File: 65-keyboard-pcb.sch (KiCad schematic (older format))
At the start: 153 parts, among them J1 USB4085-GF-A_REVA, SW1 SW_PUSH, U1 ATmega32U4-AU, X1 XTAL_GND

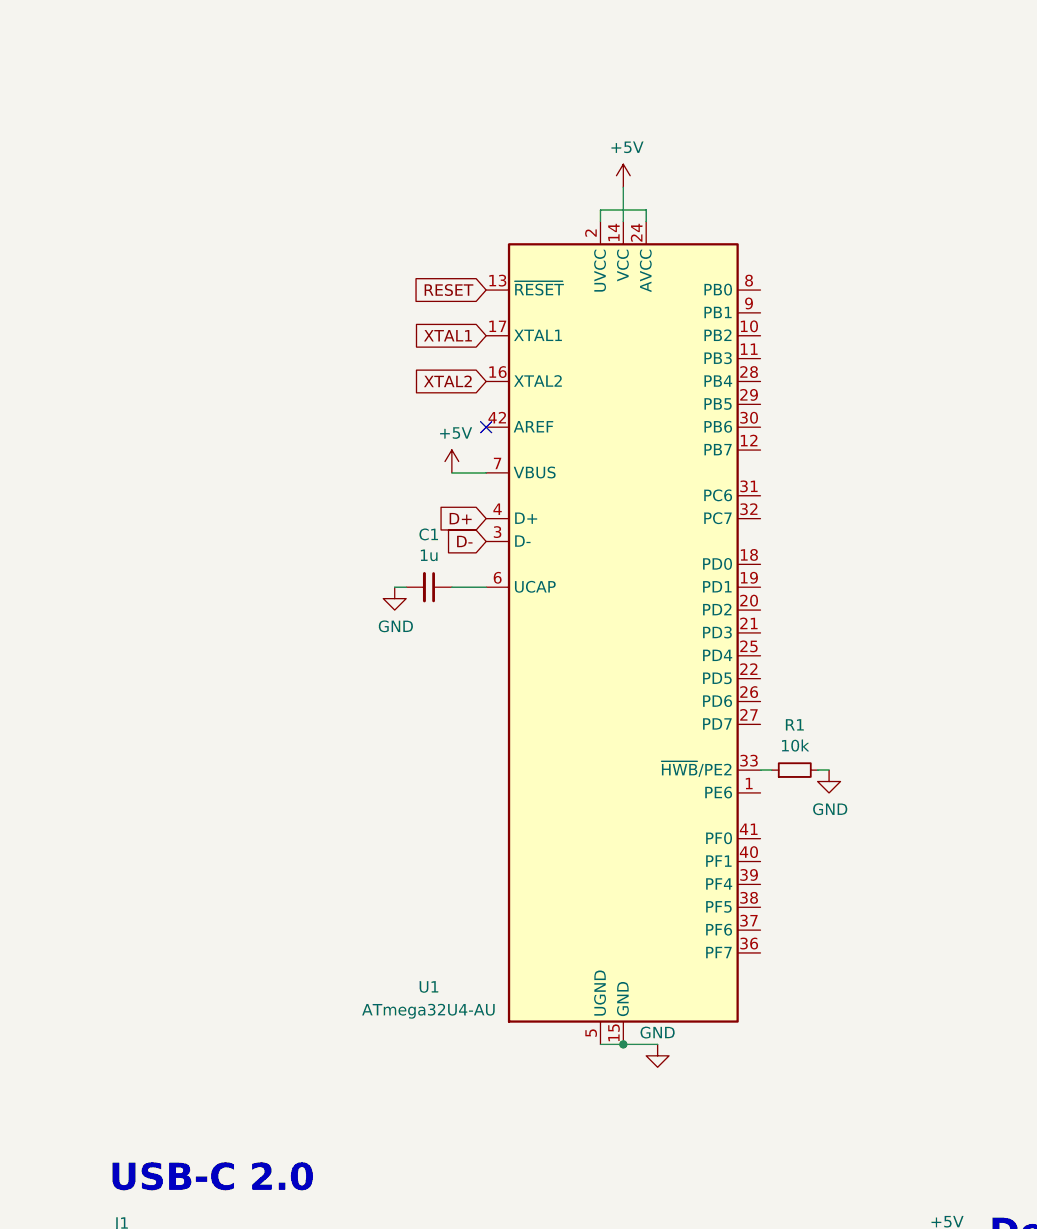
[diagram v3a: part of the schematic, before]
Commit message: Component placement
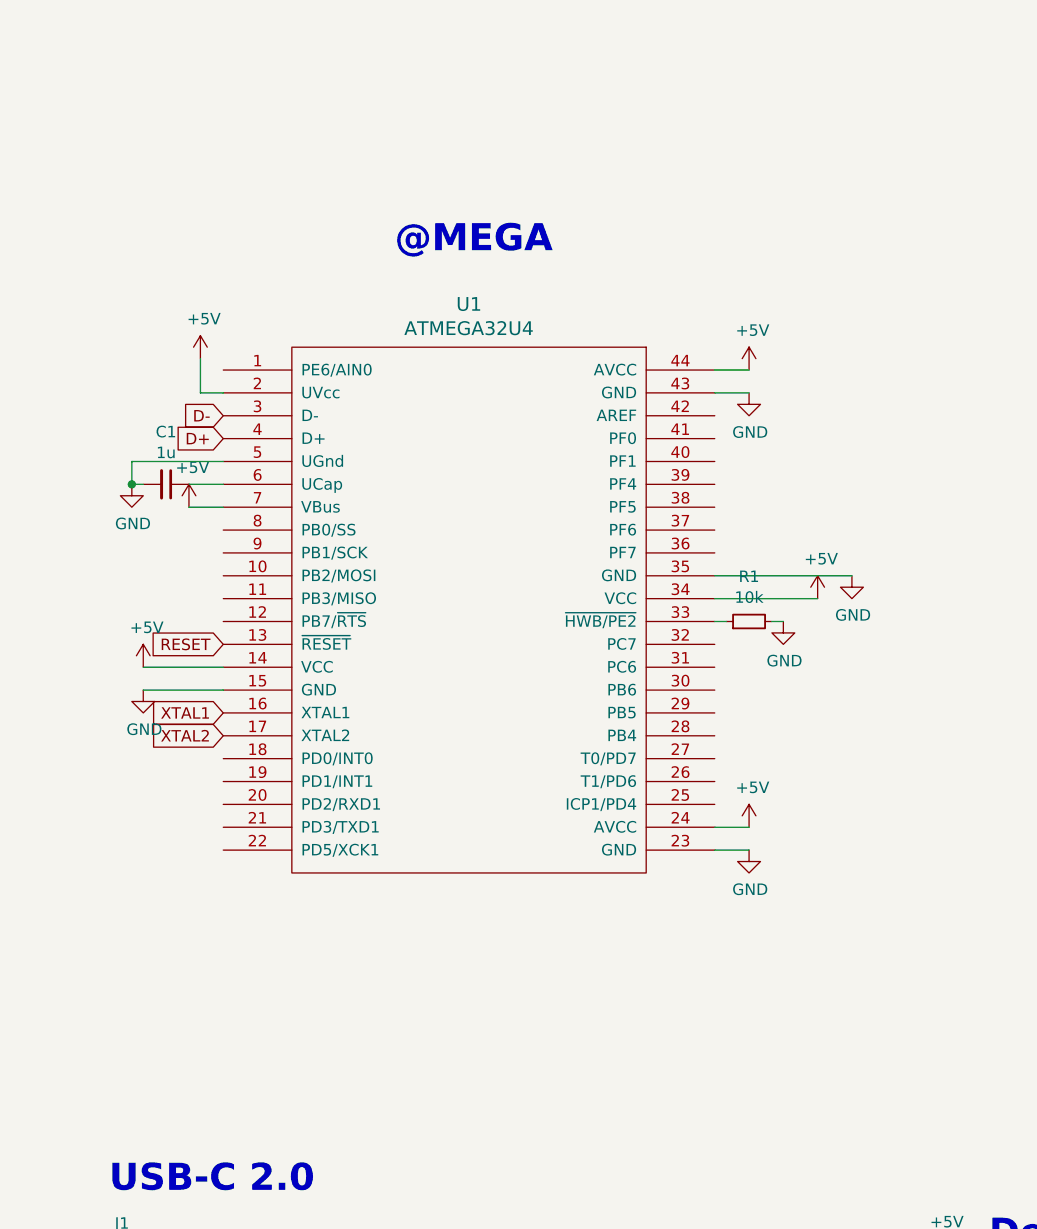
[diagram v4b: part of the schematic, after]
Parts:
- removed U1: ATmega32U4-AU, Package_QFP:TQFP-44_10x10mm_P0.8mm, symbol MCU_Microchip_ATmega:ATmega32U4-AU
- added U1: ATMEGA32U4, Package_QFP:TQFP-44_10x10mm_P0.8mm, symbol keyboard_parts:ATMEGA32U4
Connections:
- net +5V: now also U1.14 (VCC), U1.2 (UVcc), U1.24 (AVCC), U1.34 (VCC), U1.44 (AVCC), U1.7 (VBus)
- net D+: now also U1.4 (D+)
- net D-: now also U1.3 (D-)
- net GND: now also U1.15 (GND), U1.23 (GND), U1.35 (GND), U1.43 (GND), U1.5 (UGnd)
- net RESET: now also U1.13 (~RESET)
- net XTAL1: now also U1.16 (XTAL1)
- net XTAL2: now also U1.17 (XTAL2)
- net at R1.1: now also U1.33 (~HWB/PE2)
- net at C1.1: now also U1.6 (UCap)
- no-connect marks 3 -> 2
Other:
- note added: "@MEGA"
- moved on the sheet: C1, R1
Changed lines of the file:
@@
 Text GLabel 5600 4750 0    50   Input ~ 0
 ROW4
-$Comp
-L MCU_Microchip_ATmega:ATmega32U4-AU U1
-U 1 1 5F5682CF
-P 3450 3250
-F 0 "U1" H 2600 1700 50  0000 C CNN
-F 1 "ATmega32U4-AU" H 2600 1600 50  0000 C CNN
-F 2 "Package_QFP:TQFP-44_10x10mm_P0.8mm" H 3450 3250 50  0001 C CIN
-F 3 "http://ww1.microchip.com/downloads/en/DeviceDoc/Atmel-7766-8-bit-AVR-ATmega16U4-32U4_Datasheet.pdf" H 3450 3250 50  0001 C CNN
-	1    3450 3250
-	1    0    0    -1
-$EndComp
-Text GLabel 2850 1750 0    50   Input ~ 0
+Text GLabel 1700 3300 0    50   Input ~ 0
 RESET
 Text GLabel 6050 7350 2    50   Input ~ 0
@@
 $EndComp
 $Comp
-L power:GND #PWR0103
-U 1 1 5F57B366
-P 3600 5050
-F 0 "#PWR0103" H 3600 4800 50  0001 C CNN
-F 1 "GND" H 3600 5100 50  0000 C CNN
-F 2 "" H 3600 5050 50  0001 C CNN
-F 3 "" H 3600 5050 50  0001 C CNN
-	1    3600 5050
-	1    0    0    -1
-$EndComp
-Wire Wire Line
-	3350 5050 3450 5050
-Connection ~ 3450 5050
-Wire Wire Line
-	3450 5050 3600 5050
-Wire Wire Line
-	3350 1450 3350 1400
-Wire Wire Line
-	3350 1400 3550 1400
-Wire Wire Line
-	3550 1400 3550 1450
-$Comp
 L power:+5V #PWR0104
 U 1 1 5F588B35
-P 3450 1300
-F 0 "#PWR0104" H 3450 1150 50  0001 C CNN
-F 1 "+5V" H 3465 1473 50  0000 C CNN
-F 2 "" H 3450 1300 50  0001 C CNN
-F 3 "" H 3450 1300 50  0001 C CNN
-	1    3450 1300
-	1    0    0    -1
-$EndComp
-Wire Wire Line
-	3450 1300 3450 1450
+P 1600 2050
+F 0 "#PWR0104" H 1600 1900 50  0001 C CNN
+F 1 "+5V" H 1615 2223 50  0000 C CNN
+F 2 "" H 1600 2050 50  0001 C CNN
+F 3 "" H 1600 2050 50  0001 C CNN
+	1    1600 2050
+	1    0    0    -1
+$EndComp
+Wire Wire Line
+	1600 2050 1600 2200
 $Comp
 L keyboard_parts:XTAL_GND X1
@@
 Text GLabel 4300 7000 1    50   Input ~ 0
 XTAL2
-Text GLabel 2850 1950 0    50   Input ~ 0
+Text GLabel 1700 3600 0    50   Input ~ 0
 XTAL1
-Text GLabel 2850 2150 0    50   Input ~ 0
+Text GLabel 1700 3700 0    50   Input ~ 0
 XTAL2
-NoConn ~ 2850 2350
 $Comp
 L power:+5V #PWR0106
 U 1 1 5F5B165B
-P 2700 2550
-F 0 "#PWR0106" H 2700 2400 50  0001 C CNN
-F 1 "+5V" H 2715 2723 50  0000 C CNN
-F 2 "" H 2700 2550 50  0001 C CNN
-F 3 "" H 2700 2550 50  0001 C CNN
-	1    2700 2550
-	1    0    0    -1
-$EndComp
-Wire Wire Line
-	2700 2550 2850 2550
-Text GLabel 2850 2750 0    50   Input ~ 0
+P 1550 2700
+F 0 "#PWR0106" H 1550 2550 50  0001 C CNN
+F 1 "+5V" H 1565 2873 50  0000 C CNN
+F 2 "" H 1550 2700 50  0001 C CNN
+F 3 "" H 1550 2700 50  0001 C CNN
+	1    1550 2700
+	1    0    0    -1
+$EndComp
+Wire Wire Line
+	1550 2700 1700 2700
+Text GLabel 1700 2400 0    50   Input ~ 0
 D+
-Text GLabel 2850 2850 0    50   Input ~ 0
+Text GLabel 1700 2300 0    50   Input ~ 0
 D-
 $Comp
 L Device:R_Small R1
 U 1 1 5F5B953F
-P 4200 3850
-F 0 "R1" V 4396 3850 50  0000 C CNN
-F 1 "10k" V 4305 3850 50  0000 C CNN
-F 2 "Resistor_SMD:R_0805_2012Metric_Pad1.15x1.40mm_HandSolder" H 4200 3850 50  0001 C CNN
-F 3 "~" H 4200 3850 50  0001 C CNN
-	1    4200 3850
+P 4000 3200
+F 0 "R1" V 4196 3200 50  0000 C CNN
+F 1 "10k" V 4105 3200 50  0000 C CNN
+F 2 "Resistor_SMD:R_0805_2012Metric_Pad1.15x1.40mm_HandSolder" H 4000 3200 50  0001 C CNN
+F 3 "~" H 4000 3200 50  0001 C CNN
+	1    4000 3200
 	0    -1   -1   0
 $EndComp
 Wire Wire Line
-	4100 3850 4050 3850
+	3900 3200 3850 3200
 $Comp
 L power:GND #PWR0107
 U 1 1 5F5C1E45
-P 4350 3850
-F 0 "#PWR0107" H 4350 3600 50  0001 C CNN
-F 1 "GND" H 4355 3677 50  0000 C CNN
-F 2 "" H 4350 3850 50  0001 C CNN
-F 3 "" H 4350 3850 50  0001 C CNN
-	1    4350 3850
-	1    0    0    -1
-$EndComp
-Wire Wire Line
-	4350 3850 4300 3850
+P 4150 3200
+F 0 "#PWR0107" H 4150 2950 50  0001 C CNN
+F 1 "GND" H 4155 3027 50  0000 C CNN
+F 2 "" H 4150 3200 50  0001 C CNN
+F 3 "" H 4150 3200 50  0001 C CNN
+	1    4150 3200
+	1    0    0    -1
+$EndComp
+Wire Wire Line
+	4150 3200 4100 3200
 $Comp
 L Device:C_Small C1
 U 1 1 5F5CAA76
-P 2600 3050
-F 0 "C1" V 2371 3050 50  0000 C CNN
-F 1 "1u" V 2462 3050 50  0000 C CNN
-F 2 "Capacitor_SMD:C_0805_2012Metric_Pad1.15x1.40mm_HandSolder" H 2600 3050 50  0001 C CNN
-F 3 "~" H 2600 3050 50  0001 C CNN
-	1    2600 3050
+P 1450 2600
+F 0 "C1" V 1221 2600 50  0000 C CNN
+F 1 "1u" V 1312 2600 50  0000 C CNN
+F 2 "Capacitor_SMD:C_0805_2012Metric_Pad1.15x1.40mm_HandSolder" H 1450 2600 50  0001 C CNN
+F 3 "~" H 1450 2600 50  0001 C CNN
+	1    1450 2600
 	0    1    1    0
 $EndComp
@@
 L power:GND #PWR0108
 U 1 1 5F5DFA66
-P 2450 3050
-F 0 "#PWR0108" H 2450 2800 50  0001 C CNN
-F 1 "GND" H 2455 2877 50  0000 C CNN
-F 2 "" H 2450 3050 50  0001 C CNN
-F 3 "" H 2450 3050 50  0001 C CNN
-	1    2450 3050
-	1    0    0    -1
-$EndComp
-Wire Wire Line
-	2450 3050 2500 3050
-Wire Wire Line
-	2700 3050 2850 3050
+P 1300 2600
+F 0 "#PWR0108" H 1300 2350 50  0001 C CNN
+F 1 "GND" H 1305 2427 50  0000 C CNN
+F 2 "" H 1300 2600 50  0001 C CNN
+F 3 "" H 1300 2600 50  0001 C CNN
+	1    1300 2600
+	1    0    0    -1
+$EndComp
+Wire Wire Line
+	1300 2600 1350 2600
+Wire Wire Line
+	1550 2600 1700 2600
 Text Notes 3700 6600 0    118  ~ 24
 Crystal
@@
 Wire Wire Line
 	10600 2100 10600 4350
+$Comp
+L keyboard_parts:ATMEGA32U4 U1
+U 1 1 5F56E3DD
+P 2750 3150
+F 0 "U1" H 2775 4487 60  0000 C CNN
+F 1 "ATMEGA32U4" H 2775 4381 60  0000 C CNN
+F 2 "Package_QFP:TQFP-44_10x10mm_P0.8mm" H 2750 3150 60  0001 C CNN
+F 3 "" H 2750 3150 60  0000 C CNN
+	1    2750 3150
+	1    0    0    -1
+$EndComp
+Wire Wire Line
+	1700 2200 1600 2200
+$Comp
+L power:+5V #PWR0103
+U 1 1 5F5A8F73
+P 1350 3400
+F 0 "#PWR0103" H 1350 3250 50  0001 C CNN
+F 1 "+5V" H 1365 3573 50  0000 C CNN
+F 2 "" H 1350 3400 50  0001 C CNN
+F 3 "" H 1350 3400 50  0001 C CNN
+	1    1350 3400
+	1    0    0    -1
+$EndComp
+$Comp
+L power:GND #PWR0116
+U 1 1 5F5AA002
+P 1350 3500
+F 0 "#PWR0116" H 1350 3250 50  0001 C CNN
+F 1 "GND" H 1355 3327 50  0000 C CNN
+F 2 "" H 1350 3500 50  0001 C CNN
+F 3 "" H 1350 3500 50  0001 C CNN
+	1    1350 3500
+	1    0    0    -1
+$EndComp
+Wire Wire Line
+	1350 3500 1700 3500
+Wire Wire Line
+	1700 3400 1350 3400
+Wire Wire Line
+	1700 2500 1300 2500
+Wire Wire Line
+	1300 2500 1300 2600
+Connection ~ 1300 2600
+Text Notes 2450 1600 0    118  ~ 24
+@MEGA
+$Comp
+L power:+5V #PWR?
+U 1 1 5F61FD1D
+P 4000 2100
+F 0 "#PWR?" H 4000 1950 50  0001 C CNN
+F 1 "+5V" H 4015 2273 50  0000 C CNN
+F 2 "" H 4000 2100 50  0001 C CNN
+F 3 "" H 4000 2100 50  0001 C CNN
+	1    4000 2100
+	1    0    0    -1
+$EndComp
+$Comp
+L power:GND #PWR?
+U 1 1 5F620425
+P 4000 2200
+F 0 "#PWR?" H 4000 1950 50  0001 C CNN
+F 1 "GND" H 4005 2027 50  0000 C CNN
+F 2 "" H 4000 2200 50  0001 C CNN
+F 3 "" H 4000 2200 50  0001 C CNN
+	1    4000 2200
+	1    0    0    -1
+$EndComp
+Wire Wire Line
+	4000 2200 3850 2200
+Wire Wire Line
+	4000 2100 3850 2100
+$Comp
+L power:GND #PWR?
+U 1 1 5F635EFD
+P 4450 3000
+F 0 "#PWR?" H 4450 2750 50  0001 C CNN
+F 1 "GND" H 4455 2827 50  0000 C CNN
+F 2 "" H 4450 3000 50  0001 C CNN
+F 3 "" H 4450 3000 50  0001 C CNN
+	1    4450 3000
+	1    0    0    -1
+$EndComp
+$Comp
+L power:+5V #PWR?
+U 1 1 5F636303
+P 4300 3100
+F 0 "#PWR?" H 4300 2950 50  0001 C CNN
+F 1 "+5V" H 4315 3273 50  0000 C CNN
+F 2 "" H 4300 3100 50  0001 C CNN
+F 3 "" H 4300 3100 50  0001 C CNN
+	1    4300 3100
+	1    0    0    -1
+$EndComp
+Wire Wire Line
+	4300 3100 3850 3100
+Wire Wire Line
+	3850 3000 4450 3000
+$Comp
+L power:+5V #PWR?
+U 1 1 5F64C6D1
+P 4000 4100
+F 0 "#PWR?" H 4000 3950 50  0001 C CNN
+F 1 "+5V" H 4015 4273 50  0000 C CNN
+F 2 "" H 4000 4100 50  0001 C CNN
+F 3 "" H 4000 4100 50  0001 C CNN
+	1    4000 4100
+	1    0    0    -1
+$EndComp
+$Comp
+L power:GND #PWR?
+U 1 1 5F64CD40
+P 4000 4200
+F 0 "#PWR?" H 4000 3950 50  0001 C CNN
+F 1 "GND" H 4005 4027 50  0000 C CNN
+F 2 "" H 4000 4200 50  0001 C CNN
+F 3 "" H 4000 4200 50  0001 C CNN
+	1    4000 4200
+	1    0    0    -1
+$EndComp
+Wire Wire Line
+	4000 4200 3850 4200
+Wire Wire Line
+	3850 4100 4000 4100
 $EndSCHEMATC

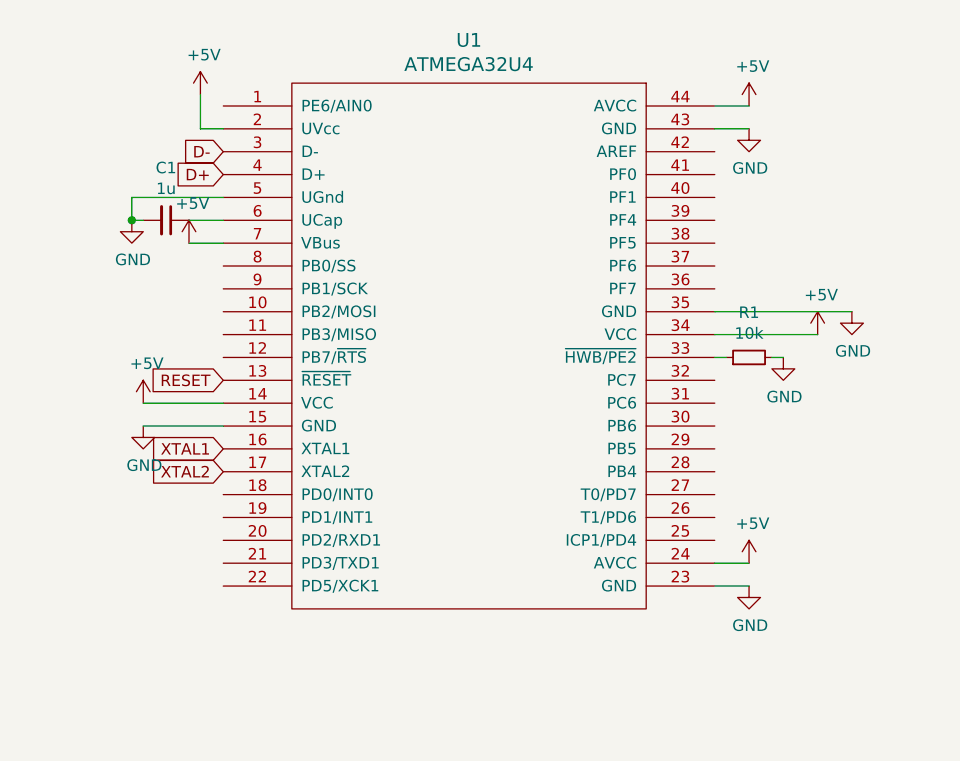
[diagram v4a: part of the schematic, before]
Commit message: Route traces
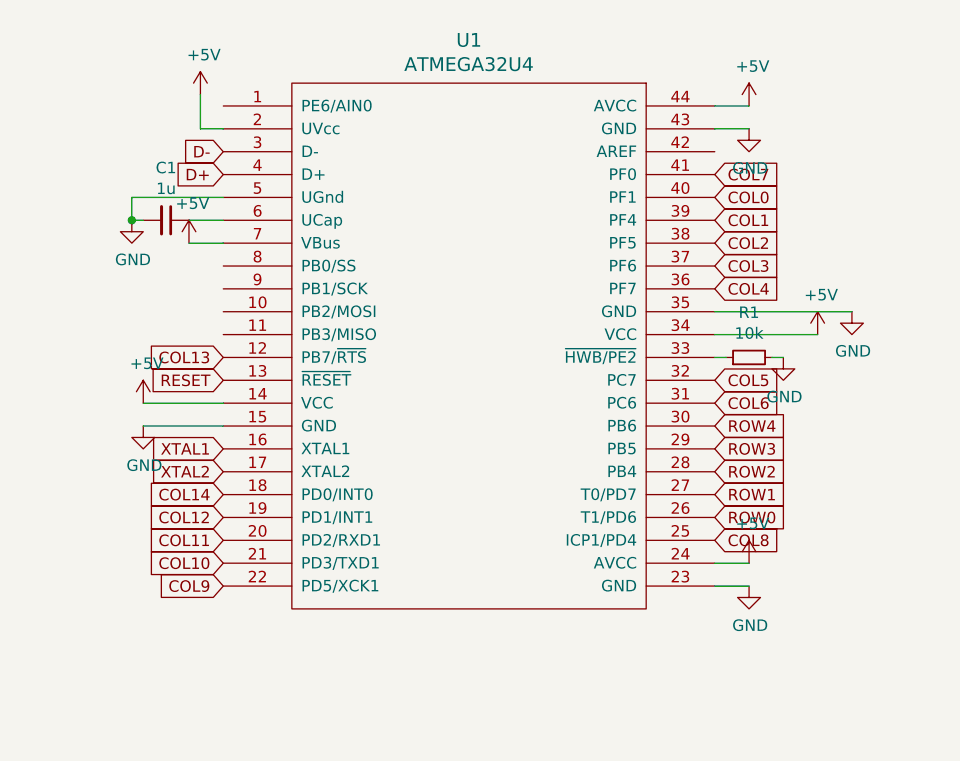
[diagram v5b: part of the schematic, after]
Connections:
- net COL0: now also U1.40 (PF1)
- net COL1: now also U1.39 (PF4)
- net COL10: now also U1.21 (PD3/TXD1)
- net COL11: now also U1.20 (PD2/RXD1)
- net COL12: now also U1.19 (PD1/INT1)
- net COL13: now also U1.12 (PB7/~RTS)
- net COL14: now also U1.18 (PD0/INT0)
- net COL2: now also U1.38 (PF5)
- net COL3: now also U1.37 (PF6)
- net COL4: now also U1.36 (PF7)
- net COL5: now also U1.32 (PC7)
- net COL6: now also U1.31 (PC6)
- net COL7: now also U1.41 (PF0)
- net COL8: now also U1.25 (ICP1/PD4)
- net COL9: now also U1.22 (PD5/XCK1)
- net ROW0: now also U1.26 (T1/PD6)
- net ROW1: now also U1.27 (T0/PD7)
- net ROW2: now also U1.28 (PB4)
- net ROW3: now also U1.29 (PB5)
- net ROW4: now also U1.30 (PB6)
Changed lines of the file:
@@
 Wire Wire Line
 	3850 4100 4000 4100
+Text GLabel 3850 3500 2    50   Input ~ 0
+ROW4
+Text GLabel 3850 3600 2    50   Input ~ 0
+ROW3
+Text GLabel 3850 3800 2    50   Input ~ 0
+ROW1
+Text GLabel 3850 3900 2    50   Input ~ 0
+ROW0
+Text GLabel 3850 2400 2    50   Input ~ 0
+COL7
+Text GLabel 3850 3400 2    50   Input ~ 0
+COL6
+Text GLabel 3850 3300 2    50   Input ~ 0
+COL5
+Text GLabel 3850 2900 2    50   Input ~ 0
+COL4
+Text GLabel 3850 2800 2    50   Input ~ 0
+COL3
+Text GLabel 3850 2700 2    50   Input ~ 0
+COL2
+Text GLabel 3850 3700 2    50   Input ~ 0
+ROW2
+Text GLabel 3850 2600 2    50   Input ~ 0
+COL1
+Text GLabel 3850 2500 2    50   Input ~ 0
+COL0
+Text GLabel 3850 4000 2    50   Input ~ 0
+COL8
+Text GLabel 1700 4200 0    50   Input ~ 0
+COL9
+Text GLabel 1700 4100 0    50   Input ~ 0
+COL10
+Text GLabel 1700 4000 0    50   Input ~ 0
+COL11
+Text GLabel 1700 3900 0    50   Input ~ 0
+COL12
+Text GLabel 1700 3800 0    50   Input ~ 0
+COL14
+Text GLabel 1700 3200 0    50   Input ~ 0
+COL13
 $EndSCHEMATC
